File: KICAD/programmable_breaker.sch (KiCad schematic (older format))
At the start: 38 parts

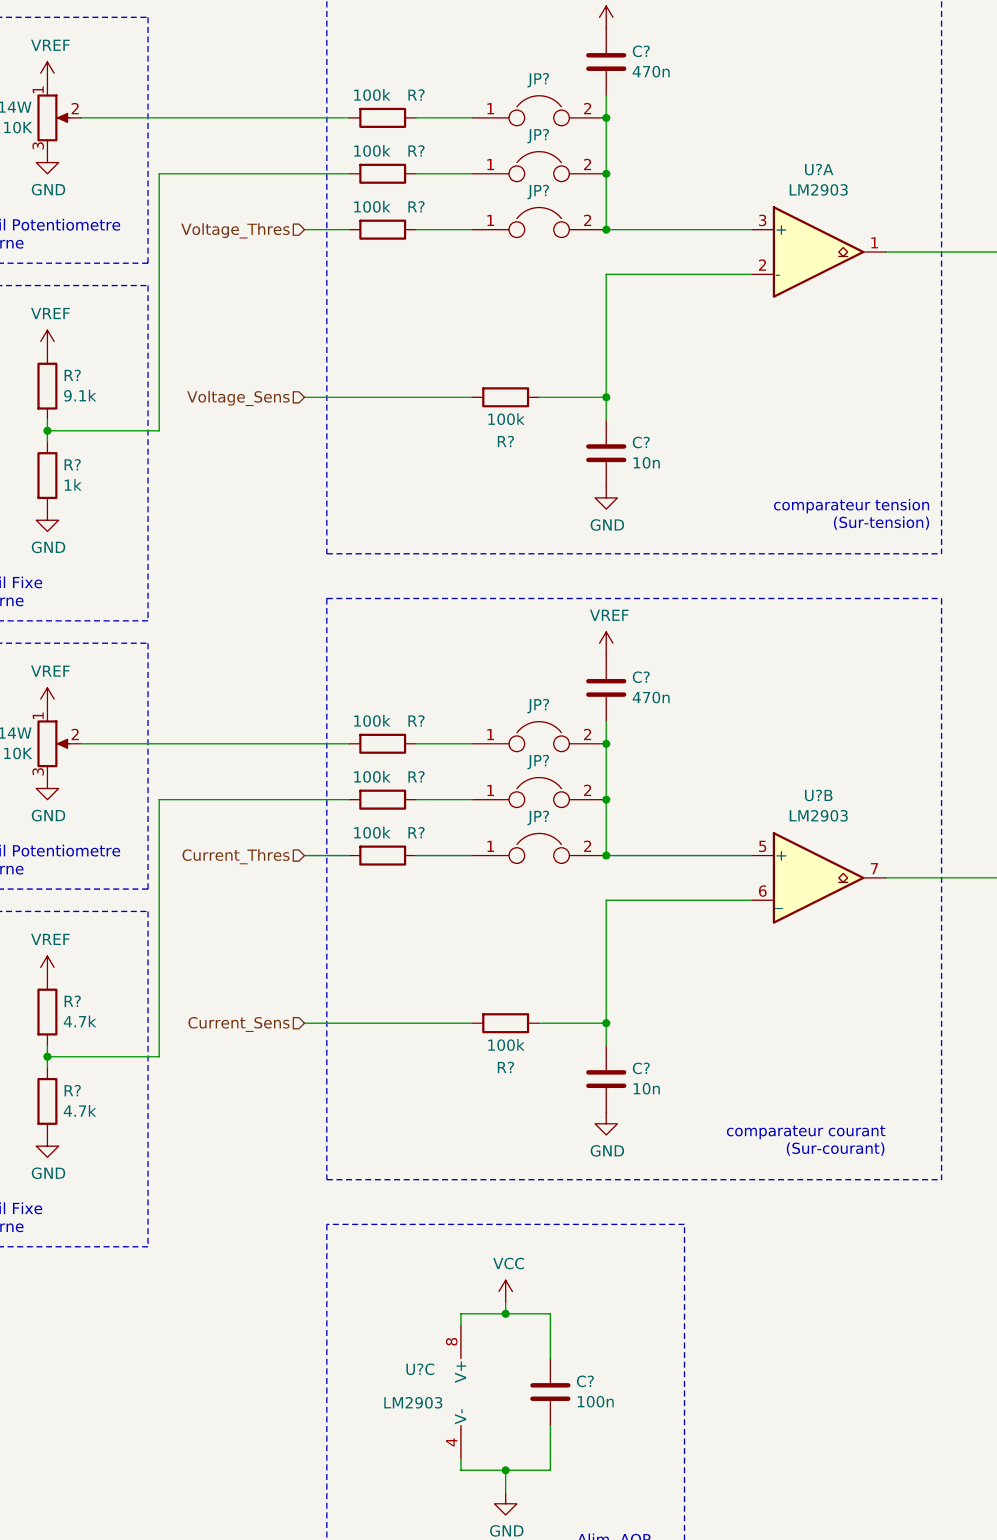
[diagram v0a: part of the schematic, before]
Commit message: minor cleanup
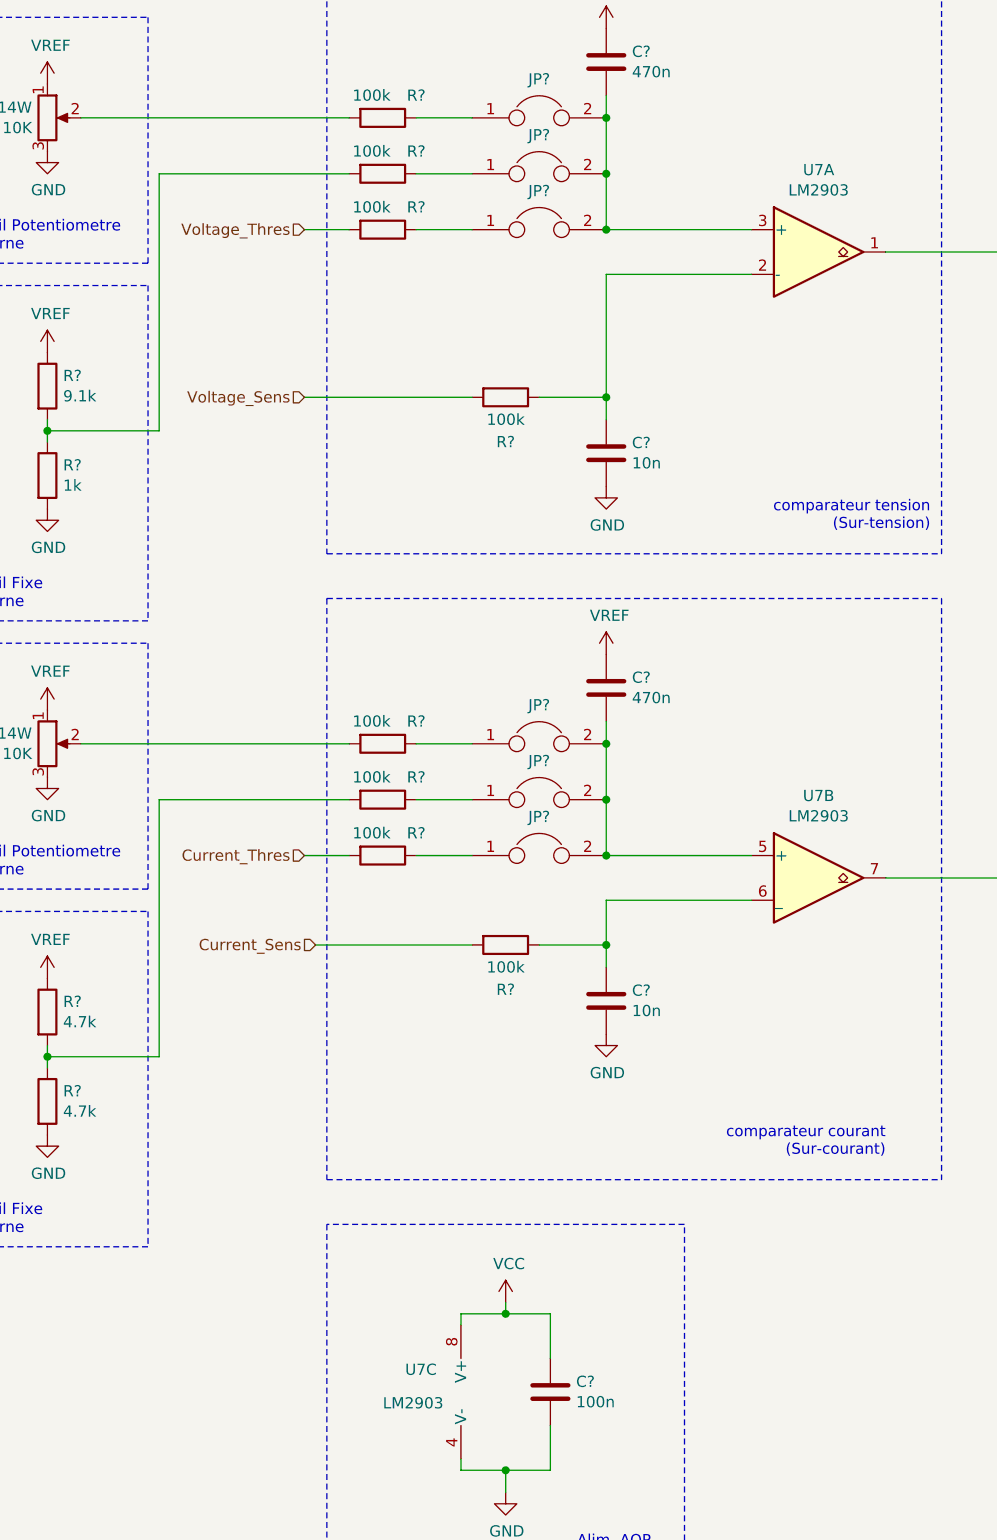
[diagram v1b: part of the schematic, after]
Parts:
- gave numbers to parts that had none: 1
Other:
- moved on the sheet: C?, R?
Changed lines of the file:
@@
 $Descr A4 11693 8268
 encoding utf-8
-Sheet 4 16
+Sheet 3 16
 Title "SESAME"
 Date ""
@@
 Text HLabel 2100 4450 0    50   Input ~ 0
 Current_Thres
-Text HLabel 2100 5200 0    50   Input ~ 0
+Text HLabel 2150 4850 0    50   Input ~ 0
 Current_Sens
 Wire Notes Line
@@
 L Device:R R?
 U 1 1 615178DC
-P 3000 5200
-F 0 "R?" V 3200 5200 50  0000 C CNN
-F 1 "100k" V 3100 5200 50  0000 C CNN
-F 2 "Resistor_SMD:R_0805_2012Metric_Pad1.20x1.40mm_HandSolder" V 2930 5200 50  0001 C CNN
-F 3 "~" H 3000 5200 50  0001 C CNN
-	1    3000 5200
+P 3000 4850
+F 0 "R?" V 3200 4850 50  0000 C CNN
+F 1 "100k" V 3100 4850 50  0000 C CNN
+F 2 "Resistor_SMD:R_0805_2012Metric_Pad1.20x1.40mm_HandSolder" V 2930 4850 50  0001 C CNN
+F 3 "~" H 3000 4850 50  0001 C CNN
+	1    3000 4850
 	0    1    1    0
 $EndComp
@@
 L Device:C C?
 U 1 1 615178FE
-P 3450 5450
-F 0 "C?" H 3565 5496 50  0000 L CNN
-F 1 "10n" H 3565 5405 50  0000 L CNN
-F 2 "Capacitor_SMD:C_0805_2012Metric_Pad1.15x1.40mm_HandSolder" H 3488 5300 50  0001 C CNN
-F 3 "~" H 3450 5450 50  0001 C CNN
-	1    3450 5450
-	1    0    0    -1
-$EndComp
-Wire Wire Line
-	3450 4650 3450 5200
+P 3450 5100
+F 0 "C?" H 3565 5146 50  0000 L CNN
+F 1 "10n" H 3565 5055 50  0000 L CNN
+F 2 "Capacitor_SMD:C_0805_2012Metric_Pad1.15x1.40mm_HandSolder" H 3488 4950 50  0001 C CNN
+F 3 "~" H 3450 5100 50  0001 C CNN
+	1    3450 5100
+	1    0    0    -1
+$EndComp
+Wire Wire Line
+	3450 4650 3450 4850
 $Comp
 L power:GND #PWR0151
 U 1 1 61517905
-P 3450 5600
-F 0 "#PWR0151" H 3450 5350 50  0001 C CNN
-F 1 "GND" H 3455 5427 50  0000 C CNN
-F 2 "" H 3450 5600 50  0001 C CNN
-F 3 "" H 3450 5600 50  0001 C CNN
-	1    3450 5600
+P 3450 5250
+F 0 "#PWR0151" H 3450 5000 50  0001 C CNN
+F 1 "GND" H 3455 5077 50  0000 C CNN
+F 2 "" H 3450 5250 50  0001 C CNN
+F 3 "" H 3450 5250 50  0001 C CNN
+	1    3450 5250
 	1    0    0    -1
 $EndComp
@@
 $EndComp
 Wire Wire Line
-	3450 5200 3150 5200
-Connection ~ 3450 5200
-Wire Wire Line
-	3450 5200 3450 5300
+	3450 4850 3150 4850
+Connection ~ 3450 4850
+Wire Wire Line
+	3450 4850 3450 4950
 Wire Wire Line
 	2100 4450 2300 4450
 Wire Wire Line
-	2100 5200 2850 5200
+	2150 4850 2850 4850
 Wire Notes Line
 	2200 3300 4950 3300
@@
 	1400 4700 1400 6200
 $Comp
-L Comparator:LM2903 U?
+L Comparator:LM2903 U7
 U 1 1 611D87A4
 P 4400 1750
-F 0 "U?" H 4400 2117 50  0000 C CNN
+F 0 "U7" H 4400 2117 50  0000 C CNN
 F 1 "LM2903" H 4400 2026 50  0000 C CNN
 F 2 "Package_SO:SOIC-8-1EP_3.9x4.9mm_P1.27mm_EP2.29x3mm" H 4400 1750 50  0001 C CNN
@@
 	4700 1750 5450 1750
 $Comp
-L Comparator:LM2903 U?
+L Comparator:LM2903 U7
 U 2 1 611EA33A
 P 4400 4550
-F 0 "U?" H 4400 4917 50  0000 C CNN
+F 0 "U7" H 4400 4917 50  0000 C CNN
 F 1 "LM2903" H 4400 4826 50  0000 C CNN
 F 2 "Package_SO:SOIC-8-1EP_3.9x4.9mm_P1.27mm_EP2.29x3mm" H 4400 4550 50  0001 C CNN
@@
 	5450 4550 6850 4550
 $Comp
-L Comparator:LM2903 U?
+L Comparator:LM2903 U7
 U 3 1 6120EB61
 P 2900 6850
-F 0 "U?" H 2550 6950 50  0000 L CNN
+F 0 "U7" H 2550 6950 50  0000 L CNN
 F 1 "LM2903" H 2450 6800 50  0000 L CNN
 F 2 "Package_SO:SOIC-8-1EP_3.9x4.9mm_P1.27mm_EP2.29x3mm" H 2900 6850 50  0001 C CNN
